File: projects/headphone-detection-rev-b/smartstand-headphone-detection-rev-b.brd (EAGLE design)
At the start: 22 x 23 mm, 19 parts, among them J1 T1M-5POS, U1 VL6180XV0NR, U2 LP5907MFX-2.8, U3 BSS138, U4 BSS138

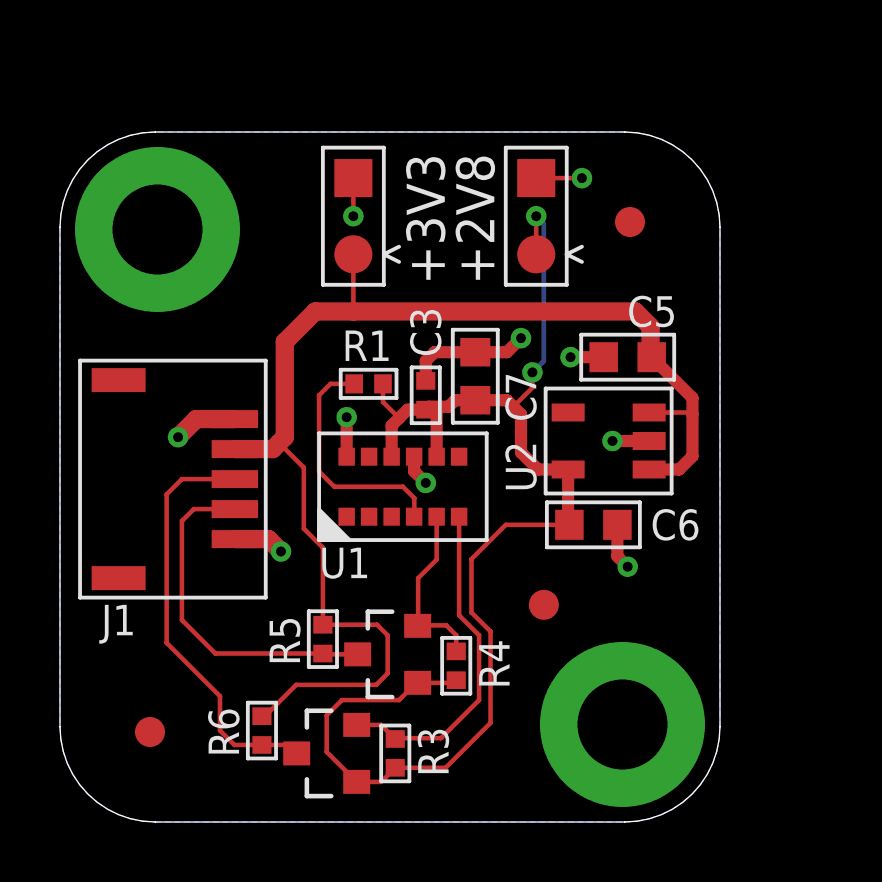
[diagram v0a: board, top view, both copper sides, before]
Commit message: Start attributizing things to help develop tooling.
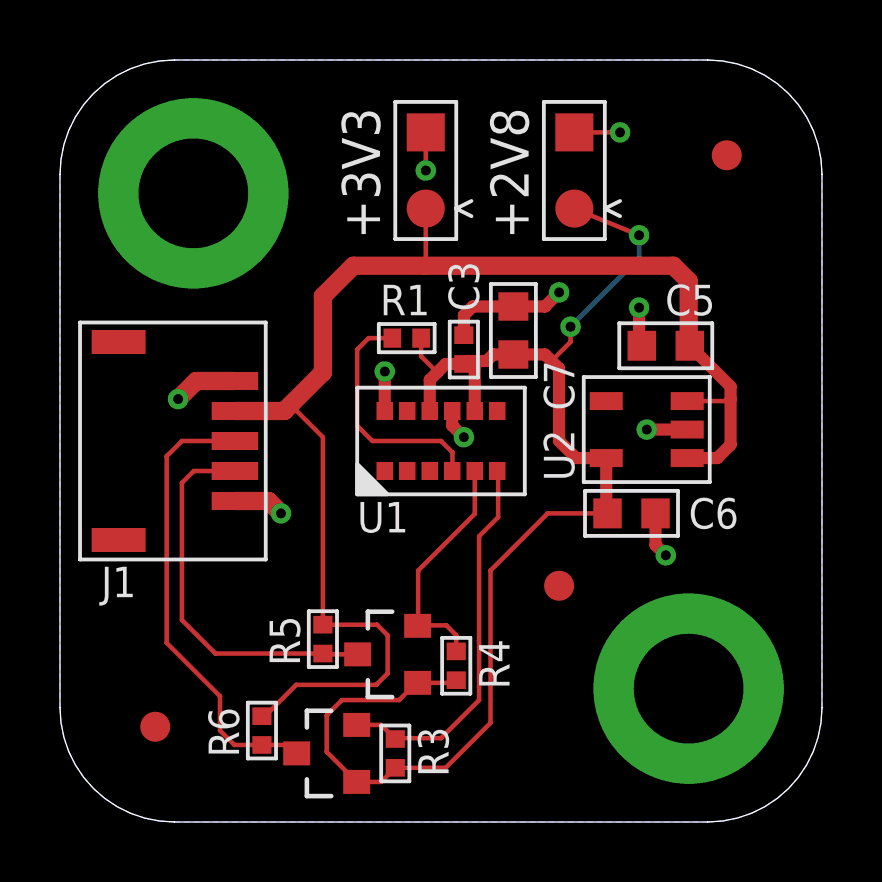
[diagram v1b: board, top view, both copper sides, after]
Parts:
- moved U$1 3.92 mm to (22.2, 22.2)
- moved TP1 2.85 mm to (12.2, 21.7)
- moved R1 1.98 mm to (11.6, 16.1)
- moved C3 1.98 mm to (13.5, 15.7)
- moved C7 1.98 mm to (15.1, 16.4)
- moved U1 1.98 mm to (12.7, 12.7)
- moved TP2 1.98 mm to (17.1, 21.7)
- moved C5 1.33 mm to (20.2, 15.9)
- moved C6 1.33 mm to (19.1, 10.3)
- moved U2 1.33 mm to (19.6, 13.1)
- moved J1 1.27 mm to (3.05, 12.7)
- moved U$3 0.81 mm to (16.6, 7.87)
- moved U$2 0.25 mm to (3.17, 3.17)
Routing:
- net +3V3: track 42.7 -> 46.1 mm
- net LOCAL_SCL: track 5.84 -> 7.89 mm
- net LOCAL_SDA: track 11.2 -> 12.7 mm
- net SDA: track 14.0 -> 15.2 mm
- net SCL: track 11.6 -> 12.8 mm
- net +2V8: track 44.2 -> 45.3 mm
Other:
- board size 22 x 23 mm -> 25.4 x 25.4 mm
